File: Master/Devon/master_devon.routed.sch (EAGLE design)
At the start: 36 parts, among them J1 ISP, K1 653002114822, K2 653002114822, K3 653002114822, K4 653002114822, U1 ATMEGA128RFA1, U2 ULN2003ADR, Y1 16MHz

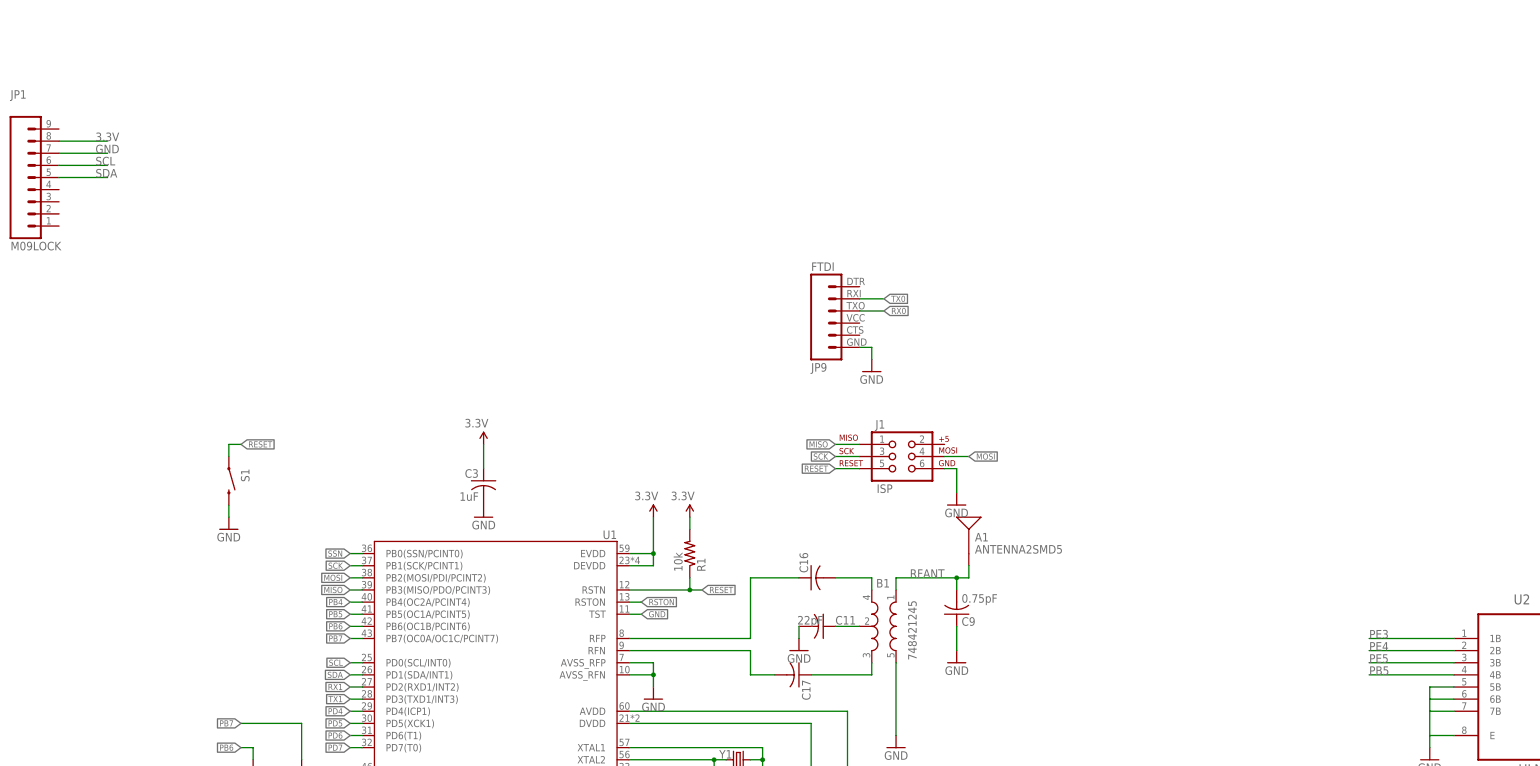
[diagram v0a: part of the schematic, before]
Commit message: Fixed main board
Hand routed some traces. Did some pin swapping. Now 2.5 x 2.5 inches.
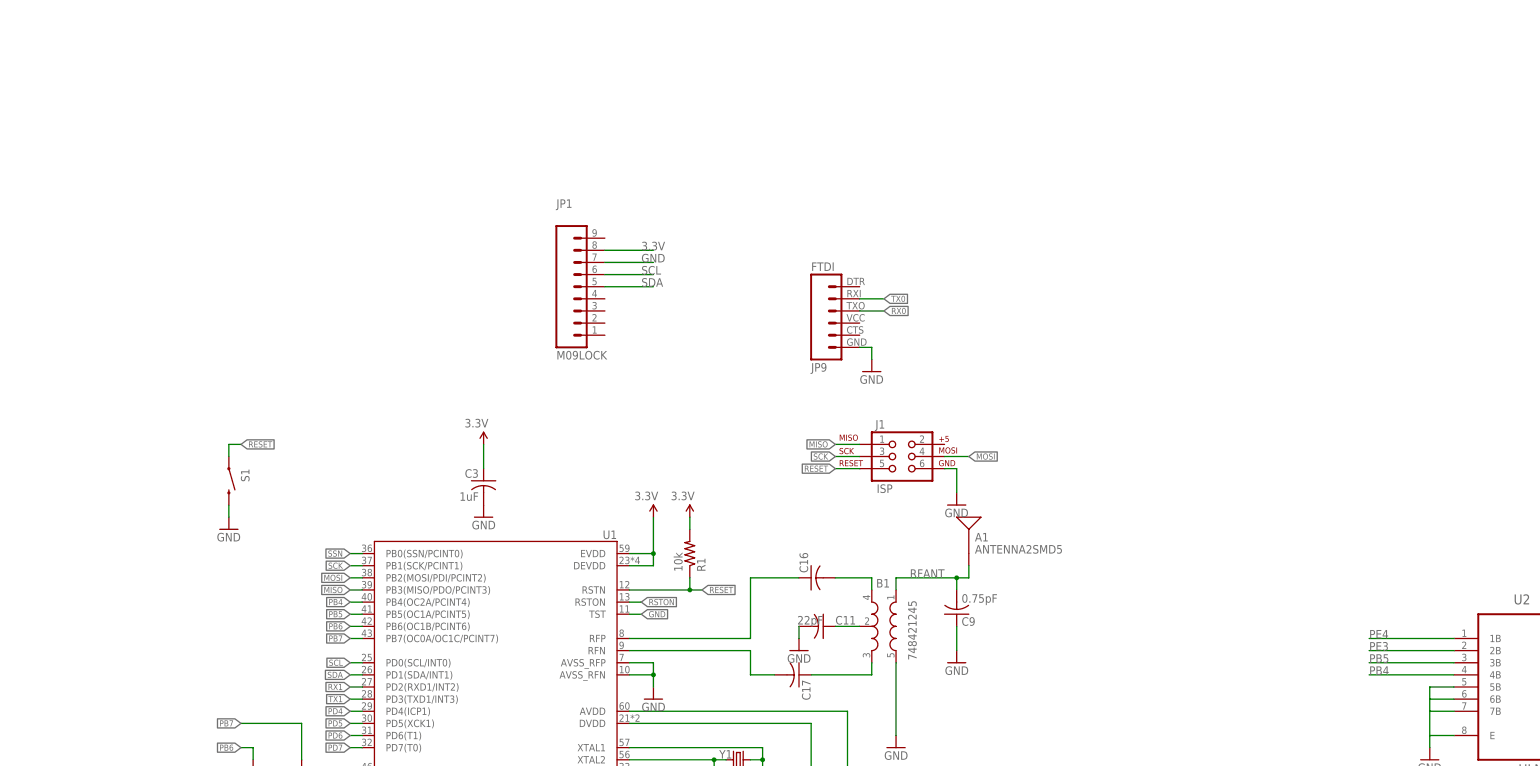
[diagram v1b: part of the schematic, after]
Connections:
- net PB4: now also U2.4B
- net PB5: now also U2.3B; no longer U2.4B
- net PE3: now also U2.2B; no longer U2.1B
- net PE4: now also U2.1B; no longer U2.2B
- net PE5: no longer U2.3B
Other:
- moved on the sheet: JP1
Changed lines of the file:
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@@
 <class number="2" name="VBATT" width="0.762" drill="0">
 </class>
-<class number="3" name="VMOTOR" width="0.2032" drill="0">
+<class number="3" name="VMOTOR" width="0.254" drill="0">
 </class>
-<class number="4" name="GND" width="0.2032" drill="0">
+<class number="4" name="GND" width="0.254" drill="0">
 </class>
 </classes>
@@
 <instance part="C10" gate="G$1" x="109.22" y="233.68"/>
 <instance part="SUPPLY1" gate="GND" x="109.22" y="223.52"/>
-<instance part="JP1" gate="G$1" x="-40.64" y="177.8"/>
+<instance part="JP1" gate="G$1" x="73.66" y="154.94"/>
 <instance part="C12" gate="G$1" x="309.88" y="114.3" rot="MR0"/>
 <instance part="C13" gate="G$1" x="337.82" y="114.3" rot="MR0"/>
@@
 </busses>
 <nets>
-<net name="GND" class="0">
+<net name="GND" class="4">
 <segment>
 <pinref part="U1" gate="G$1" pin="PADDLE"/>
@@
 <segment>
 <pinref part="JP1" gate="G$1" pin="7"/>
-<wire x1="-30.48" y1="182.88" x2="-20.32" y2="182.88" width="0.1524" layer="91"/>
-<label x="-22.86" y="182.88" size="1.778" layer="95"/>
+<wire x1="83.82" y1="160.02" x2="93.98" y2="160.02" width="0.1524" layer="91"/>
+<label x="91.44" y="160.02" size="1.778" layer="95"/>
 </segment>
 </net>
@@
 <label x="30.48" y="40.64" size="1.27" layer="95" rot="MR0" xref="yes"/>
 </segment>
-<segment>
-<pinref part="U2" gate="A" pin="3B"/>
-<wire x1="243.84" y1="76.2" x2="261.62" y2="76.2" width="0.1524" layer="91"/>
-<label x="243.84" y="76.2" size="1.778" layer="95"/>
-</segment>
 </net>
 <net name="PE4" class="0">
@@
 </segment>
 <segment>
+<pinref part="U2" gate="A" pin="1B"/>
+<wire x1="261.62" y1="81.28" x2="243.84" y2="81.28" width="0.1524" layer="91"/>
+<label x="243.84" y="81.28" size="1.778" layer="95"/>
+</segment>
+</net>
+<net name="PE3" class="0">
+<segment>
+<pinref part="U1" gate="G$1" pin="PE3(OC3A/AIN1)"/>
+<wire x1="33.02" y1="45.72" x2="30.48" y2="45.72" width="0.1524" layer="91"/>
+<label x="30.48" y="45.72" size="1.27" layer="95" rot="MR0" xref="yes"/>
+</segment>
+<segment>
 <pinref part="U2" gate="A" pin="2B"/>
 <wire x1="261.62" y1="78.74" x2="243.84" y2="78.74" width="0.1524" layer="91"/>
@@
 </segment>
 </net>
-<net name="PE3" class="0">
-<segment>
-<pinref part="U1" gate="G$1" pin="PE3(OC3A/AIN1)"/>
-<wire x1="33.02" y1="45.72" x2="30.48" y2="45.72" width="0.1524" layer="91"/>
-<label x="30.48" y="45.72" size="1.27" layer="95" rot="MR0" xref="yes"/>
-</segment>
-<segment>
-<pinref part="U2" gate="A" pin="1B"/>
-<wire x1="243.84" y1="81.28" x2="261.62" y2="81.28" width="0.1524" layer="91"/>
-<label x="243.84" y="81.28" size="1.778" layer="95"/>
-</segment>
-</net>
 <net name="PE2" class="0">
 <segment>
@@
 <segment>
 <pinref part="JP1" gate="G$1" pin="5"/>
-<wire x1="-30.48" y1="177.8" x2="-20.32" y2="177.8" width="0.1524" layer="91"/>
-<label x="-22.86" y="177.8" size="1.778" layer="95"/>
+<wire x1="83.82" y1="154.94" x2="93.98" y2="154.94" width="0.1524" layer="91"/>
+<label x="91.44" y="154.94" size="1.778" layer="95"/>
 </segment>
 </net>
@@
 <segment>
 <pinref part="JP1" gate="G$1" pin="6"/>
-<wire x1="-30.48" y1="180.34" x2="-20.32" y2="180.34" width="0.1524" layer="91"/>
-<label x="-22.86" y="180.34" size="1.778" layer="95"/>
+<wire x1="83.82" y1="157.48" x2="93.98" y2="157.48" width="0.1524" layer="91"/>
+<label x="91.44" y="157.48" size="1.778" layer="95"/>
 </segment>
 </net>
@@
 </segment>
 <segment>
-<pinref part="U2" gate="A" pin="4B"/>
-<wire x1="243.84" y1="73.66" x2="261.62" y2="73.66" width="0.1524" layer="91"/>
-<label x="243.84" y="73.66" size="1.778" layer="95"/>
+<pinref part="U2" gate="A" pin="3B"/>
+<wire x1="261.62" y1="76.2" x2="243.84" y2="76.2" width="0.1524" layer="91"/>
+<label x="243.84" y="76.2" size="1.778" layer="95"/>
 </segment>
 </net>
@@
 <wire x1="33.02" y1="88.9" x2="30.48" y2="88.9" width="0.1524" layer="91"/>
 <label x="30.48" y="88.9" size="1.27" layer="95" rot="MR0" xref="yes"/>
+</segment>
+<segment>
+<pinref part="U2" gate="A" pin="4B"/>
+<wire x1="261.62" y1="73.66" x2="243.84" y2="73.66" width="0.1524" layer="91"/>
+<label x="243.84" y="73.66" size="1.778" layer="95"/>
 </segment>
 </net>
@@
 <segment>
 <pinref part="JP1" gate="G$1" pin="8"/>
-<wire x1="-30.48" y1="185.42" x2="-20.32" y2="185.42" width="0.1524" layer="91"/>
-<label x="-22.86" y="185.42" size="1.778" layer="95"/>
+<wire x1="83.82" y1="162.56" x2="93.98" y2="162.56" width="0.1524" layer="91"/>
+<label x="91.44" y="162.56" size="1.778" layer="95"/>
 </segment>
 </net>
@@
 </segment>
 </net>
-<net name="VBATT" class="3">
+<net name="VBATT" class="2">
 <segment>
 <pinref part="U2" gate="A" pin="COM"/>

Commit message: Revert "Fixed main board"
This reverts commit e8d481ade4fad3f727996ef615af2e559dd81647.
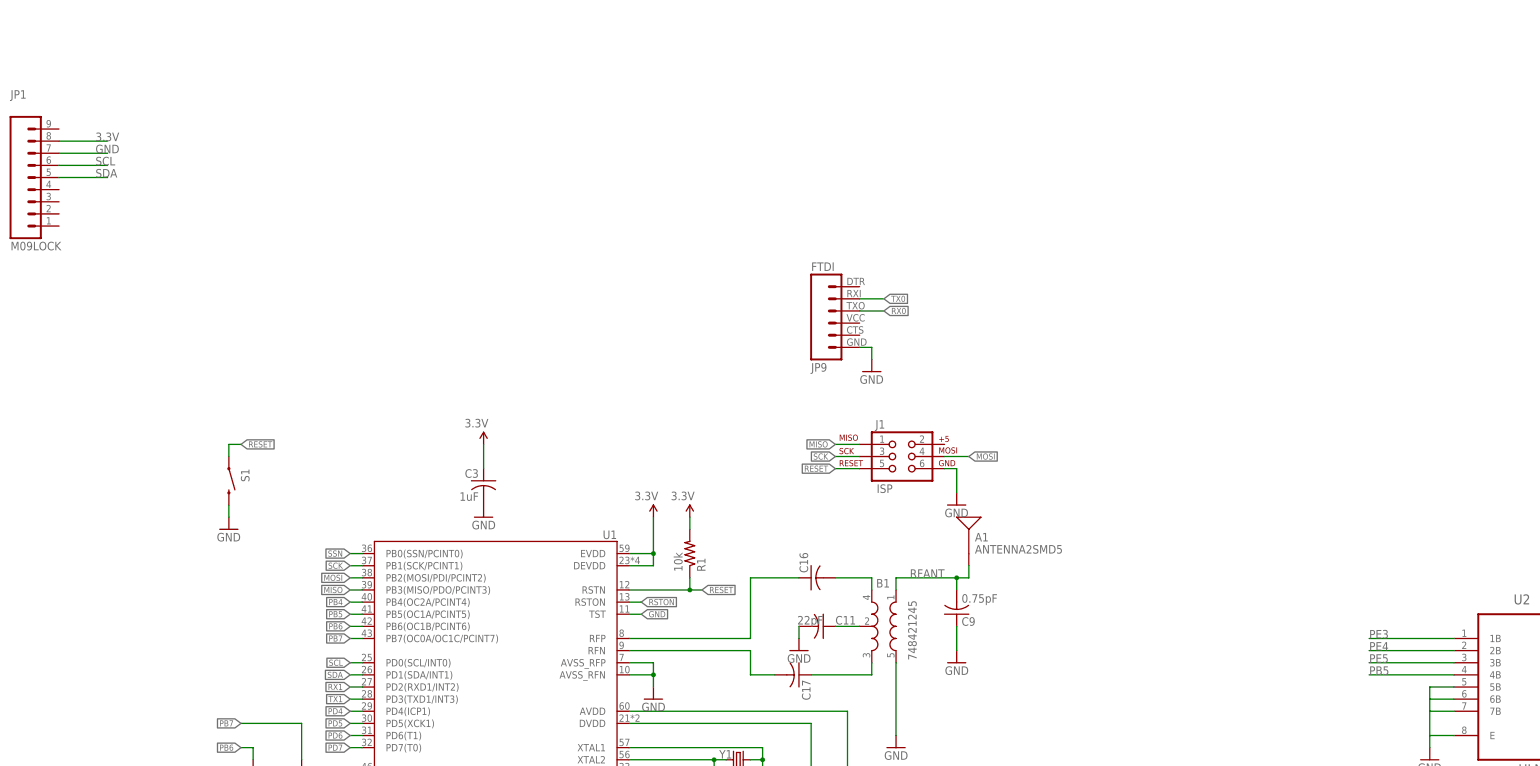
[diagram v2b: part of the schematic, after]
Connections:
- net PB4: no longer U2.4B
- net PB5: now also U2.4B; no longer U2.3B
- net PE3: now also U2.1B; no longer U2.2B
- net PE4: now also U2.2B; no longer U2.1B
- net PE5: now also U2.3B
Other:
- moved on the sheet: JP1
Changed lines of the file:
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@@
 <class number="2" name="VBATT" width="0.762" drill="0">
 </class>
-<class number="3" name="VMOTOR" width="0.254" drill="0">
+<class number="3" name="VMOTOR" width="0.2032" drill="0">
 </class>
-<class number="4" name="GND" width="0.254" drill="0">
+<class number="4" name="GND" width="0.2032" drill="0">
 </class>
 </classes>
@@
 <instance part="C10" gate="G$1" x="109.22" y="233.68"/>
 <instance part="SUPPLY1" gate="GND" x="109.22" y="223.52"/>
-<instance part="JP1" gate="G$1" x="73.66" y="154.94"/>
+<instance part="JP1" gate="G$1" x="-40.64" y="177.8"/>
 <instance part="C12" gate="G$1" x="309.88" y="114.3" rot="MR0"/>
 <instance part="C13" gate="G$1" x="337.82" y="114.3" rot="MR0"/>
@@
 </busses>
 <nets>
-<net name="GND" class="4">
+<net name="GND" class="0">
 <segment>
 <pinref part="U1" gate="G$1" pin="PADDLE"/>
@@
 <segment>
 <pinref part="JP1" gate="G$1" pin="7"/>
-<wire x1="83.82" y1="160.02" x2="93.98" y2="160.02" width="0.1524" layer="91"/>
-<label x="91.44" y="160.02" size="1.778" layer="95"/>
+<wire x1="-30.48" y1="182.88" x2="-20.32" y2="182.88" width="0.1524" layer="91"/>
+<label x="-22.86" y="182.88" size="1.778" layer="95"/>
 </segment>
 </net>
@@
 <label x="30.48" y="40.64" size="1.27" layer="95" rot="MR0" xref="yes"/>
 </segment>
+<segment>
+<pinref part="U2" gate="A" pin="3B"/>
+<wire x1="243.84" y1="76.2" x2="261.62" y2="76.2" width="0.1524" layer="91"/>
+<label x="243.84" y="76.2" size="1.778" layer="95"/>
+</segment>
 </net>
 <net name="PE4" class="0">
@@
 </segment>
 <segment>
-<pinref part="U2" gate="A" pin="1B"/>
-<wire x1="261.62" y1="81.28" x2="243.84" y2="81.28" width="0.1524" layer="91"/>
-<label x="243.84" y="81.28" size="1.778" layer="95"/>
+<pinref part="U2" gate="A" pin="2B"/>
+<wire x1="261.62" y1="78.74" x2="243.84" y2="78.74" width="0.1524" layer="91"/>
+<label x="243.84" y="78.74" size="1.778" layer="95"/>
 </segment>
 </net>
@@
 </segment>
 <segment>
-<pinref part="U2" gate="A" pin="2B"/>
-<wire x1="261.62" y1="78.74" x2="243.84" y2="78.74" width="0.1524" layer="91"/>
-<label x="243.84" y="78.74" size="1.778" layer="95"/>
+<pinref part="U2" gate="A" pin="1B"/>
+<wire x1="243.84" y1="81.28" x2="261.62" y2="81.28" width="0.1524" layer="91"/>
+<label x="243.84" y="81.28" size="1.778" layer="95"/>
 </segment>
 </net>
@@
 <segment>
 <pinref part="JP1" gate="G$1" pin="5"/>
-<wire x1="83.82" y1="154.94" x2="93.98" y2="154.94" width="0.1524" layer="91"/>
-<label x="91.44" y="154.94" size="1.778" layer="95"/>
+<wire x1="-30.48" y1="177.8" x2="-20.32" y2="177.8" width="0.1524" layer="91"/>
+<label x="-22.86" y="177.8" size="1.778" layer="95"/>
 </segment>
 </net>
@@
 <segment>
 <pinref part="JP1" gate="G$1" pin="6"/>
-<wire x1="83.82" y1="157.48" x2="93.98" y2="157.48" width="0.1524" layer="91"/>
-<label x="91.44" y="157.48" size="1.778" layer="95"/>
+<wire x1="-30.48" y1="180.34" x2="-20.32" y2="180.34" width="0.1524" layer="91"/>
+<label x="-22.86" y="180.34" size="1.778" layer="95"/>
 </segment>
 </net>
@@
 </segment>
 <segment>
-<pinref part="U2" gate="A" pin="3B"/>
-<wire x1="261.62" y1="76.2" x2="243.84" y2="76.2" width="0.1524" layer="91"/>
-<label x="243.84" y="76.2" size="1.778" layer="95"/>
+<pinref part="U2" gate="A" pin="4B"/>
+<wire x1="243.84" y1="73.66" x2="261.62" y2="73.66" width="0.1524" layer="91"/>
+<label x="243.84" y="73.66" size="1.778" layer="95"/>
 </segment>
 </net>
@@
 <wire x1="33.02" y1="88.9" x2="30.48" y2="88.9" width="0.1524" layer="91"/>
 <label x="30.48" y="88.9" size="1.27" layer="95" rot="MR0" xref="yes"/>
-</segment>
-<segment>
-<pinref part="U2" gate="A" pin="4B"/>
-<wire x1="261.62" y1="73.66" x2="243.84" y2="73.66" width="0.1524" layer="91"/>
-<label x="243.84" y="73.66" size="1.778" layer="95"/>
 </segment>
 </net>
@@
 <segment>
 <pinref part="JP1" gate="G$1" pin="8"/>
-<wire x1="83.82" y1="162.56" x2="93.98" y2="162.56" width="0.1524" layer="91"/>
-<label x="91.44" y="162.56" size="1.778" layer="95"/>
+<wire x1="-30.48" y1="185.42" x2="-20.32" y2="185.42" width="0.1524" layer="91"/>
+<label x="-22.86" y="185.42" size="1.778" layer="95"/>
 </segment>
 </net>
@@
 </segment>
 </net>
-<net name="VBATT" class="2">
+<net name="VBATT" class="3">
 <segment>
 <pinref part="U2" gate="A" pin="COM"/>
